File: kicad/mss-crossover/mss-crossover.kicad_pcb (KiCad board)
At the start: 2 copper layers, 76.2 x 57.2 mm, 64 parts, among them J1 Screw_Terminal_01x02, J10 SM04B-SRSS, J2 Screw_Terminal_01x02, J3 Screw_Terminal_01x02, J4 Screw_Terminal_01x02, J5 690-005-299-043, J6 SM04B-SRSS, J7 Micro_SD_Card_Det_Hirose_DM3AT, J8 Screw_Terminal_01x02, J9 Conn_01x05, SW1 FSM4JSMATR, SW2 FSM4JSMATR, U1 AP63203WU, U2 ESP32-S2-SOLO, U3 MAX98357AETE+T

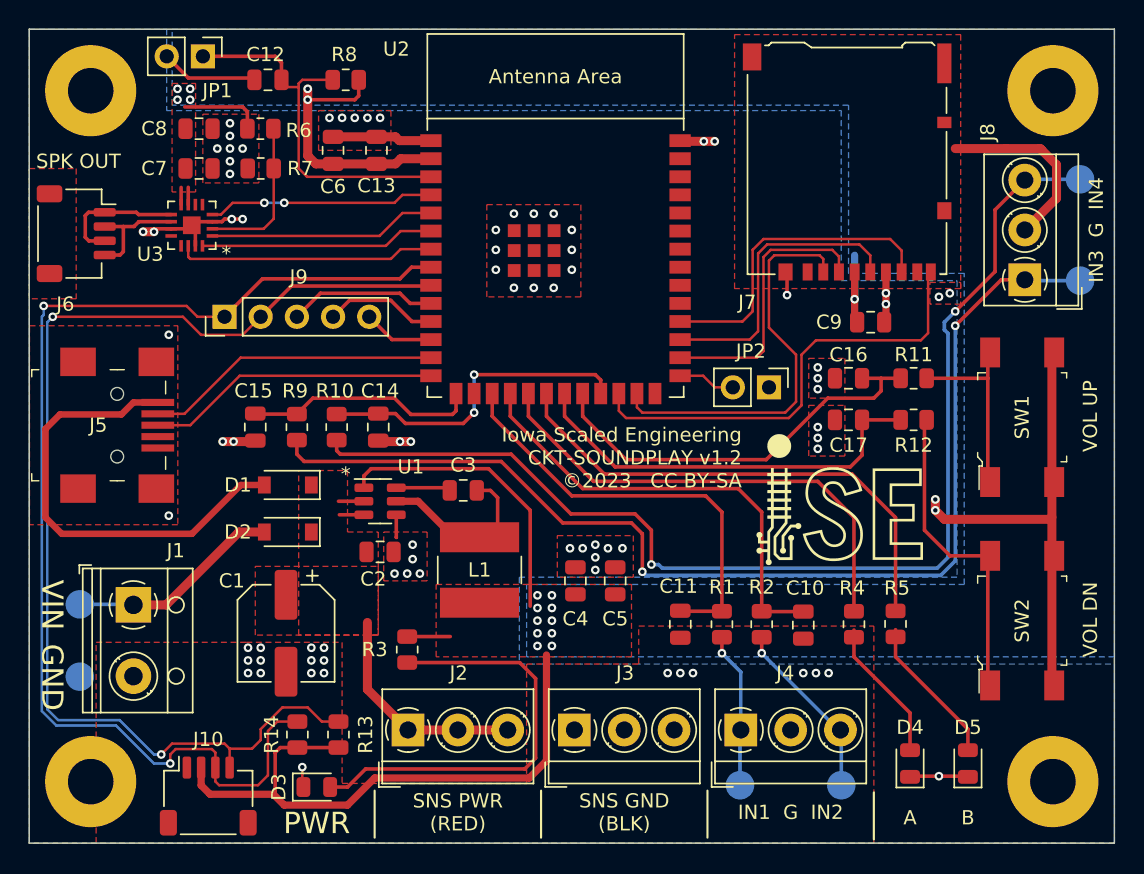
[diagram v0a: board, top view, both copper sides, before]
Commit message: Initial PCB layout complete on v2.0
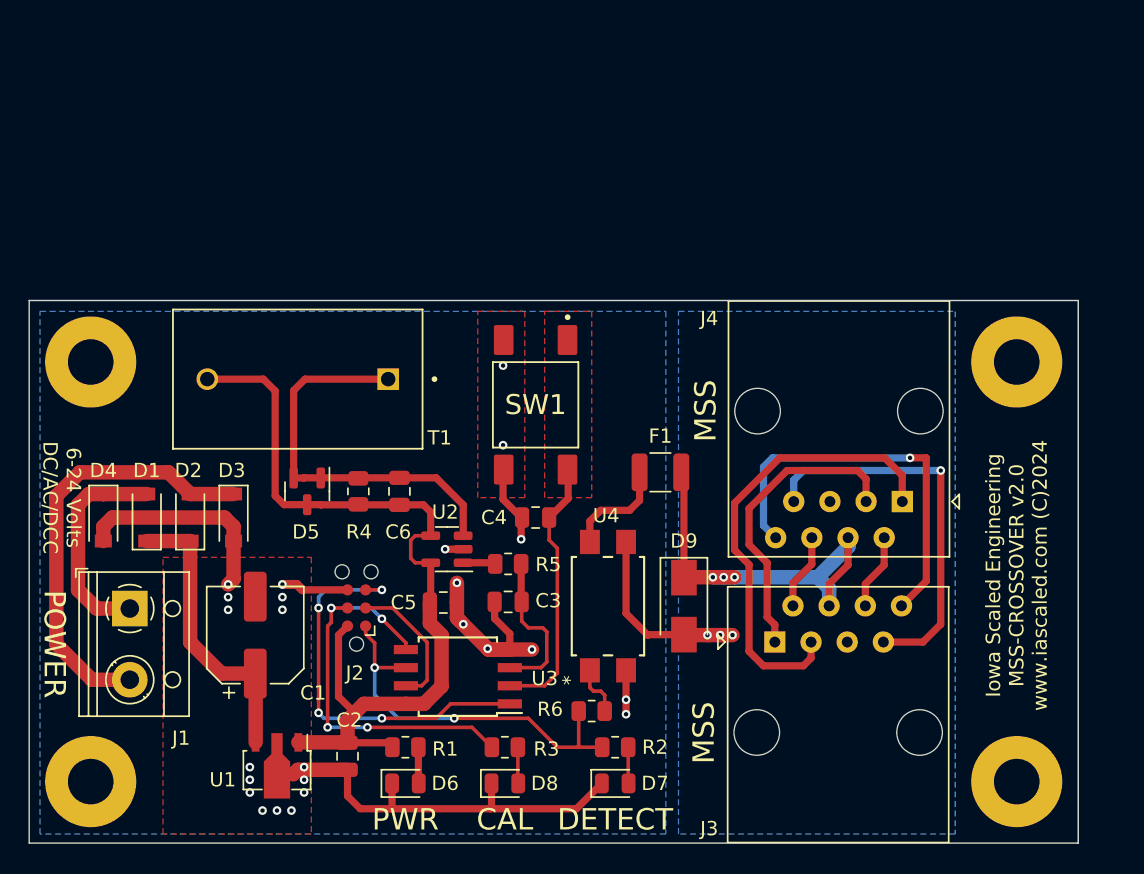
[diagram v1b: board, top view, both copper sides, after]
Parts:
- removed C10, C11, C12, C14, C15, C16, C17: 1uF, Capacitor_SMD:C_0805_2012Metric
- removed C13, C7, C9: 0.1uF, Capacitor_SMD:C_0805_2012Metric
- removed C8: 10uF, Capacitor_SMD:C_0805_2012Metric
- removed J10, J6: SM04B-SRSS, Connector_JST:JST_SH_SM04B-SRSS-TB_1x04-1MP_P1.00mm_Horizontal
- removed J5: 690-005-299-043, digikey-footprints:USB_Mini_B_Female_690-005-299-043
- removed J7: Micro_SD_Card_Det_Hirose_DM3AT, Connector_Card:microSD_HC_Hirose_DM3AT-SF-PEJM5
- removed J8: Screw_Terminal_01x02, TerminalBlock_MetzConnect:TerminalBlock_MetzConnect_Type059_RT06303HBWC_1x03_P3.50mm_Horizontal
- removed J9: Conn_01x05, Connector_PinHeader_2.54mm:PinHeader_1x05_P2.54mm_Vertical
- removed JP1, JP2: Conn_01x02, Connector_PinHeader_2.54mm:PinHeader_1x02_P2.54mm_Vertical
- removed L1: 4.7uH, ISE_UltraLibrarian:MSS6132-xxxMLC
- removed R10, R11, R12, R9: 1k, Resistor_SMD:R_0805_2012Metric
- removed R13, R14, R8: 10k, Resistor_SMD:R_0805_2012Metric
- removed R7: DNI, Resistor_SMD:R_0805_2012Metric
- removed SW2: FSM4JSMATR, digikey-footprints:Switch_Tactile_SMD_6x6mm
- removed TP1, TP2, TP3, TP4, TP5, TP6: TestPoint, TestPoint:TestPoint_Pad_D2.0mm
- added D6: GREEN LED, LED_SMD:LED_0805_2012Metric, F.Cu at (51.8, 187.6)
- added D7: RED LED, LED_SMD:LED_0805_2012Metric, F.Cu at (66.5, 187.6)
- added D8: AMBER LED, LED_SMD:LED_0805_2012Metric, F.Cu at (58.8, 187.6)
- added D9: SMAJ18A-TP, Diode_SMD:D_SMA, F.Cu at (71.4, 175.1)
- added F1: 1210L020WR, Resistor_SMD:R_1210_3225Metric, F.Cu at (69.7, 165.7)
- added T1: PE-51687, ISE_Generic:XFMR_PE-51687, F.Cu at (44.3, 159.2)
- added U4: TLP241A, ISE_UltraLibrarian:11-5B201S_TOS, F.Cu at (66.0, 175.1)
- C2: value 10uF -> 22uF
- C3: value 0.1uF -> 1uF
- C4, C5: value 22uF -> 0.1uF
- C6: value 10uF -> 0.1uF
- D1, D2: value D_Schottky -> CDBM140G
- D3: value GREEN LED -> CDBM140G; footprint LED_SMD:LED_0805_2012Metric -> Diode_SMD:D_SOD-123
- D4: value RED LED -> CDBM140G; footprint LED_SMD:LED_0805_2012Metric -> Diode_SMD:D_SOD-123
- D5: value RED LED -> BAV99; footprint LED_SMD:LED_0805_2012Metric -> Package_TO_SOT_SMD:SOT-23
- J2: value Screw_Terminal_01x02 -> AVR-ISP; footprint TerminalBlock_MetzConnect:TerminalBlock_MetzConnect_Type059_RT06303HBWC_1x03_P3.50mm_Horizontal -> Connector:Tag-Connect_TC2030-IDC-NL_2x03_P1.27mm_Vertical
- J3, J4: value Screw_Terminal_01x02 -> 8P8C; footprint TerminalBlock_MetzConnect:TerminalBlock_MetzConnect_Type059_RT06303HBWC_1x03_P3.50mm_Horizontal -> Connector_RJ:RJ45_Amphenol_54602-x08_Horizontal
- R3: value 330 -> 1k
- R4: value 330 -> 510
- R5: value 330 -> 100k
- R6: value DNI -> 330
- SW1: footprint digikey-footprints:Switch_Tactile_SMD_6x6mm -> ISE_Generic:TE_FSM4JSMA
- U1: value AP63203WU -> AP7381-33Y; footprint Package_TO_SOT_SMD:TSOT-23-6 -> ISE_Generic:SOT-89-3
- U2: value ESP32-S2-SOLO -> INA180A4; footprint Espressif:ESP32-S2-SOLO -> Package_TO_SOT_SMD:SOT-23-5
- U3: value MAX98357AETE+T -> ATtiny85-20S; footprint ISE_UltraLibrarian:21-0136I_T1633-4_MXM -> Package_SO:SOIC-8W_5.3x5.3mm_P1.27mm
- moved D4 59.2 mm to (30.6, 168.9), turned to -90 degrees
- moved D5 50.2 mm to (44.9, 167.1), turned to -90 degrees
- moved R6 47.0 mm to (64.9, 182.5)
- moved U3 36.8 mm to (55.5, 180.1)
- moved R4 36.0 mm to (48.5, 167.1)
- moved SW1 34.2 mm to (61.0, 161.0), turned to -90 degrees
- moved R5 27.5 mm to (59.0, 172.2), turned to 180 degrees
- moved C6 24.4 mm to (51.4, 167.1), turned to -90 degrees
- moved R1 23.8 mm to (51.8, 185.0), turned to 180 degrees
- moved U2 21.8 mm to (54.7, 171.1), turned to 180 degrees
- moved U1 19.9 mm to (42.8, 186.3), turned to -90 degrees
- moved D3 19.8 mm to (39.8, 168.9), turned to -90 degrees
- moved J4 19.6 mm to (86.7, 167.8), turned to 180 degrees
- moved H3 19.2 mm to (94.7, 158.0)
- moved H4 19.1 mm to (29.7, 158.0)
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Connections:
- C2 pad 1: /VPWR -> +3.3V
- C3 pad 1: Net-(C3-Pad1) -> /DCC_CURRENT
- C3 pad 2: Net-(C3-Pad2) -> GND
- C4 pad 1: +3.3V -> //CAL_SW
- C6 pad 1: +3.3V -> Net-(D5-Pad1)
- C6 pad 2: GND -> +3.3V
- D3 pad 1: GND -> Net-(D2-Pad2)
- D3 pad 2: Net-(D3-Pad2) -> GND
- D4 pad 1: GND -> Net-(D1-Pad2)
- D4 pad 2: Net-(D4-Pad2) -> GND
- D5 pad 1: GND -> Net-(D5-Pad1)
- D5 pad 2: Net-(D5-Pad2) -> Net-(D5-Pad1)
- J1 pad 1: Net-(D2-Pad2) -> Net-(D1-Pad2)
- J1 pad 2: GND -> Net-(D2-Pad2)
- J2 pad 1: /VPWR -> Net-(J2-Pad1)
- J2 pad 2: /VPWR -> +3.3V
- J2 pad 3: /VPWR -> Net-(J2-Pad3)
- J3 pad 1: GND -> Net-(J3-Pad1)
- J3 pad 2: GND -> Net-(J3-Pad2)
- J3 pad 3: GND -> Net-(J3-Pad3)
- J4 pad 1: Net-(J4-Pad1) -> Net-(J3-Pad3)
- J4 pad 2: GND -> Net-(J3-Pad6)
- J4 pad 3: Net-(J4-Pad3) -> Net-(J3-Pad1)
- R1 pad 1: Net-(J4-Pad1) -> Net-(D6-Pad2)
- R1 pad 2: /EN1 -> +3.3V
- R2 pad 1: Net-(J4-Pad3) -> Net-(J2-Pad1)
- R2 pad 2: /EN2 -> Net-(R2-Pad2)
- R3 pad 1: Net-(D3-Pad2) -> Net-(J2-Pad4)
- R3 pad 2: +3.3V -> Net-(R3-Pad2)
- R4 pad 1: Net-(D4-Pad2) -> +3.3V
- R4 pad 2: /LEDA -> Net-(D5-Pad1)
- R5 pad 1: Net-(D5-Pad2) -> /DCC_CURRENT
- R5 pad 2: /LEDB -> Net-(R5-Pad2)
- R6 pad 1: /GAIN_SLOT -> Net-(U4-Pad1)
- R6 pad 2: +3.3V -> Net-(J2-Pad1)
- SW1 pad 1: Net-(R11-Pad1) -> //CAL_SW
- SW1 pad 2: Net-(R11-Pad1) -> //CAL_SW
- U1 pad 2: /VPWR -> GND
- U2 pad 1: GND -> Net-(R5-Pad2)
- U2 pad 2: +3.3V -> GND
- U2 pad 3: /~{RST} -> Net-(D5-Pad1)
- U2 pad 4: /I2S_SD -> +3.3V
- U2 pad 5: /I2S_DATA -> +3.3V
- U3 pad 1: /I2S_DATA -> Net-(J2-Pad5)
- U3 pad 2: /GAIN_SLOT -> //CAL_SW
- U3 pad 3: GND -> /DCC_CURRENT
- U3 pad 4: /I2S_SD -> GND
- U3 pad 5: unconnected-(U3-Pad5) -> Net-(J2-Pad4)
- U3 pad 6: unconnected-(U3-Pad6) -> Net-(J2-Pad1)
- U3 pad 7: +3.3V -> Net-(J2-Pad3)
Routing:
- net /AUX1: track 83.6 -> 0.00 mm, vias 2 -> 0
- net /AUX2: track 81.8 -> 0.00 mm, vias 2 -> 0
- net Net-(J8-Pad3): track 81.6 -> 0.00 mm, vias 2 -> 0
- net Net-(J8-Pad1): track 79.4 -> 0.00 mm, vias 2 -> 0
- net +3.3V: track 100.5 -> 61.5 mm, vias 17 -> 0
- net /LEDB: track 35.1 -> 0.00 mm
- net /LEDA: track 33.5 -> 0.00 mm
- net Net-(J3-Pad3): track 0.00 -> 32.4 mm
- net /SDDET: track 32.1 -> 0.00 mm
- net /EN2: track 31.4 -> 0.00 mm
- net Net-(D3-Pad2): track 30.2 -> 0.00 mm
- net /EN1: track 29.8 -> 0.00 mm
- net /VOLDN: track 29.5 -> 0.00 mm
- net /MSS_OCC: track 0.00 -> 29.5 mm, vias 0 -> 3
- net /VOLUP: track 29.4 -> 0.00 mm
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- added copper zone on B.Cu, net /MSS_GND
- added copper zone on F.Cu, net //CAL_SW
- removed copper zone on B.Cu, net +3.3V
- removed copper zone on F.Cu, net +3.3V
- removed copper zone on F.Cu, net /MPJ6
- removed copper zone on F.Cu, net /VPWR
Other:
- board size 76.2 x 57.2 mm -> 73.7 x 38.1 mm
- board text added: "6-24 Volts DC/AC/DCC"
- board text added: "CAL"
- board text added: "DETECT"
- board text added: "Iowa Scaled Engineering MSS-CROSSOVER v2.0 www.iascaled.com (C)2024"
- board text added: "MSS"
- board text added: "POWER"
- board text removed: "*"
- board text removed: "A"
- board text removed: "B"
- board text removed: "GND"
- board text removed: "IN1 G IN2"
- board text removed: "IN3 G IN4"
- board text removed: "Iowa Scaled Engineering CKT-SOUNDPLAY v1.2 ©2023 CC BY-SA"
- board text removed: "SNS GND (BLK)"
- board text removed: "SNS PWR (RED)"
- board text removed: "SPK OUT"
- board text removed: "VIN"
- board text removed: "VOL DN"
- board text removed: "VOL UP"
